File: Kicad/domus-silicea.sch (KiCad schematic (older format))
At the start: 6 parts, among them U1 MCP1640

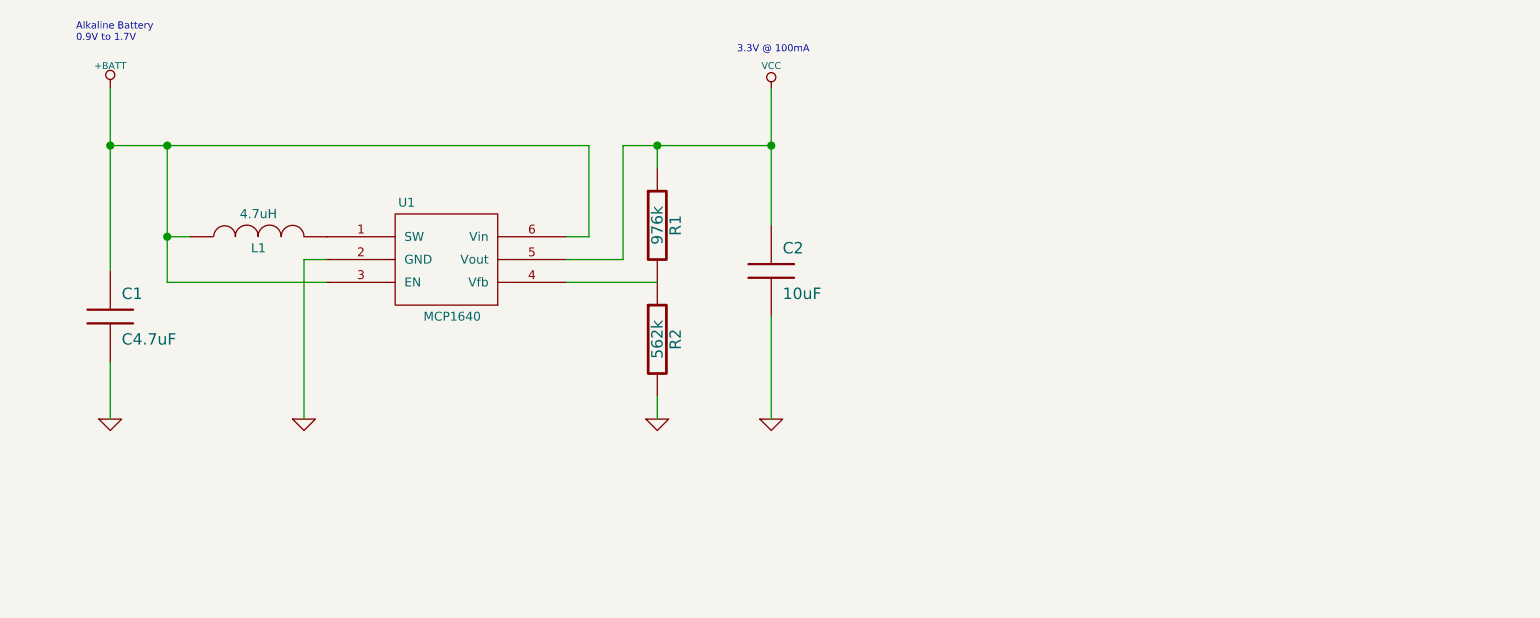
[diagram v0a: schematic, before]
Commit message: KiCad
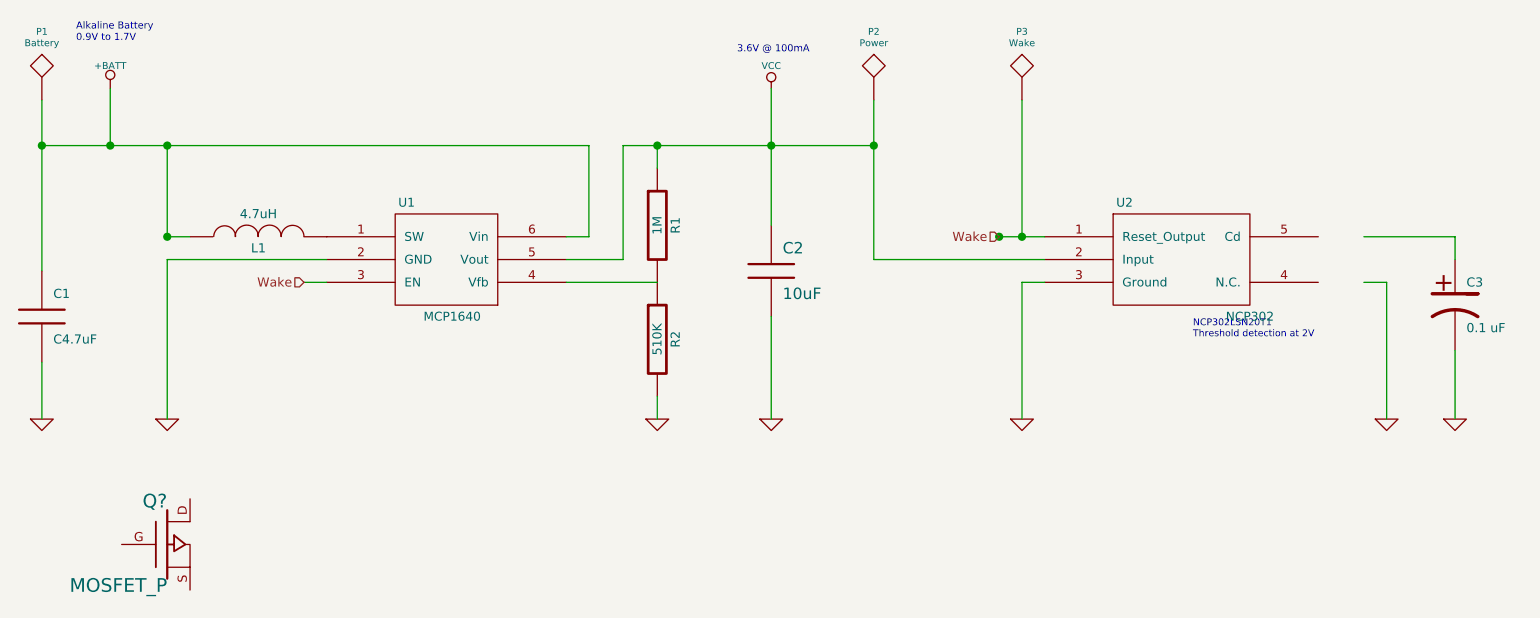
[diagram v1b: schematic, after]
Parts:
- added C3: 0.1 uF, symbol CP1
- added P1: Battery, symbol TST
- added P2: Power, symbol TST
- added P3: Wake, symbol TST
- added Q?: MOSFET_P, symbol MOSFET_P
- added U2: NCP302, symbol NCP302
- R1: value 976k -> 1M
- R2: value 562k -> 510K
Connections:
- net labels added: Wake
- wire segments 18 -> 30
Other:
- note added: "3.6V @ 100mA"
- note added: "NCP302LSN20T1\nThreshold detection at 2V"
- note removed: "3.3V @ 100mA"
- moved on the sheet: C1
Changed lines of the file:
@@
-EESchema Schematic File Version 2  date 2/13/2015 09:27:14
+EESchema Schematic File Version 2  date 2/16/2015 17:59:50
 LIBS:power
 LIBS:device
@@
 LIBS:valves
 LIBS:customComponents
-EELAYER 43  0
+LIBS:domus-silicea-cache
+EELAYER 25  0
 EELAYER END
 $Descr A4 11700 8267
@@
 Sheet 1 1
 Title "Silicino Prototype"
-Date "13 feb 2015"
+Date "16 feb 2015"
 Rev ""
 Comp ""
@@
 $EndDescr
 Wire Wire Line
-	1850 1700 1750 1700
-Wire Wire Line
-	1750 1700 1750 2400
-Wire Wire Line
-	900  2150 900  2400
+	1850 1700 1150 1700
+Connection ~ 600  1200
+Wire Wire Line
+	600  1750 600  1000
+Connection ~ 4900 1600
+Wire Wire Line
+	4900 1000 4900 1600
+Wire Wire Line
+	4250 1200 3150 1200
+Wire Wire Line
+	4250 1000 4250 1700
+Wire Wire Line
+	4250 1700 5000 1700
+Connection ~ 4800 1600
+Wire Wire Line
+	1750 1800 1850 1800
+Wire Wire Line
+	600  1200 3000 1200
+Wire Wire Line
+	4900 2400 4900 1800
+Wire Wire Line
+	4900 1800 5000 1800
+Wire Wire Line
+	6400 1600 6800 1600
+Wire Wire Line
+	6800 1600 6800 1700
+Wire Wire Line
+	1150 1700 1150 2400
+Wire Wire Line
+	600  2150 600  2400
 Connection ~ 3800 1200
 Wire Wire Line
@@
 Wire Wire Line
 	2900 1800 3300 1800
-Wire Wire Line
-	1850 1800 1150 1800
 Wire Wire Line
 	1250 1600 1150 1600
@@
 	3800 2400 3800 1950
 Connection ~ 1150 1200
-Wire Wire Line
-	1150 1800 1150 1200
 Connection ~ 900  1200
 Wire Wire Line
-	900  950  900  1750
-Wire Wire Line
 	2900 1600 3000 1600
 Wire Wire Line
 	3000 1600 3000 1200
 Wire Wire Line
-	3000 1200 900  1200
-Wire Wire Line
 	2900 1700 3150 1700
 Wire Wire Line
 	3150 1700 3150 1200
-Wire Wire Line
-	3150 1200 3800 1200
 Wire Wire Line
 	3300 1200 3300 1300
 Connection ~ 3300 1200
+Wire Wire Line
+	6800 2100 6800 2400
+Wire Wire Line
+	6500 2400 6500 1800
+Wire Wire Line
+	6500 1800 6400 1800
+Connection ~ 4250 1200
+Wire Wire Line
+	1150 1600 1150 1200
+Wire Wire Line
+	5000 1600 4800 1600
+Wire Wire Line
+	900  950  900  1200
+Text HLabel 1750 1800 0    40   Input ~ 0
+Wake
+Text HLabel 4800 1600 0    40   Input ~ 0
+Wake
+$Comp
+L MOSFET_P Q?
+U 1 1 54E2206B
+P 1150 2950
+F 0 "Q?" H 1150 3140 60  0000 R CNN
+F 1 "MOSFET_P" H 1150 2770 60  0000 R CNN
+	1    1150 2950
+	1    0    0    -1
+$EndComp
+Text Notes 5650 2050 0    30   ~ 0
+ NCP302LSN20T1\nThreshold detection at 2V
+$Comp
+L TST P1
+U 1 1 54E1F74F
+P 600 1000
+F 0 "P1" H 600 1300 30  0000 C CNN
+F 1 "Battery" H 600 1250 30  0000 C CNN
+	1    600  1000
+	1    0    0    -1
+$EndComp
+$Comp
+L TST P2
+U 1 1 54E1F73D
+P 4250 1000
+F 0 "P2" H 4250 1300 30  0000 C CNN
+F 1 "Power" H 4250 1250 30  0000 C CNN
+	1    4250 1000
+	1    0    0    -1
+$EndComp
+$Comp
+L TST P3
+U 1 1 54E1F729
+P 4900 1000
+F 0 "P3" H 4900 1300 30  0000 C CNN
+F 1 "Wake" H 4900 1250 30  0000 C CNN
+	1    4900 1000
+	1    0    0    -1
+$EndComp
+$Comp
+L CP1 C3
+U 1 1 54E1F57F
+P 6800 1900
+F 0 "C3" H 6850 2000 40  0000 L CNN
+F 1 "0.1 uF" H 6850 1800 40  0000 L CNN
+	1    6800 1900
+	1    0    0    -1
+$EndComp
+$Comp
+L GND #PWR?
+U 1 1 54E1F526
+P 6800 2400
+F 0 "#PWR?" H 6800 2400 30  0001 C CNN
+F 1 "GND" H 6800 2330 30  0001 C CNN
+	1    6800 2400
+	1    0    0    -1
+$EndComp
+$Comp
+L GND #PWR?
+U 1 1 54E1F521
+P 6500 2400
+F 0 "#PWR?" H 6500 2400 30  0001 C CNN
+F 1 "GND" H 6500 2330 30  0001 C CNN
+	1    6500 2400
+	1    0    0    -1
+$EndComp
+$Comp
+L GND #PWR?
+U 1 1 54E1F508
+P 4900 2400
+F 0 "#PWR?" H 4900 2400 30  0001 C CNN
+F 1 "GND" H 4900 2330 30  0001 C CNN
+	1    4900 2400
+	1    0    0    -1
+$EndComp
+$Comp
+L NCP302 U2
+U 1 1 54E1F4D1
+P 5350 1700
+F 0 "U2" H 5350 1950 39  0000 C CNN
+F 1 "NCP302" H 5900 1450 39  0000 C CNN
+	1    5350 1700
+	1    0    0    -1
+$EndComp
 $Comp
 L MCP1640 U1
@@
 Alkaline Battery\n0.9V to 1.7V\n
 Text Notes 3650 800  0    31   ~ 0
-3.3V @ 100mA
+3.6V @ 100mA
 $Comp
 L VCC #PWR?
@@
 L GND #PWR?
 U 1 1 54DDAFB7
-P 900 2400
-F 0 "#PWR?" H 900 2400 30  0001 C CNN
-F 1 "GND" H 900 2330 30  0001 C CNN
-	1    900  2400
+P 600 2400
+F 0 "#PWR?" H 600 2400 30  0001 C CNN
+F 1 "GND" H 600 2330 30  0001 C CNN
+	1    600  2400
 	1    0    0    -1
 $EndComp
@@
 L C C1
 U 1 1 54DDABB5
-P 900 1950
-F 0 "C1" H 950 2050 50  0000 L CNN
-F 1 "C4.7uF" H 950 1850 50  0000 L CNN
-	1    900  1950
+P 600 1950
+F 0 "C1" H 650 2050 40  0000 L CNN
+F 1 "C4.7uF" H 650 1850 40  0000 L CNN
+	1    600  1950
 	1    0    0    -1
 $EndComp
@@
 U 1 1 54DDAB61
 P 3300 2050
-F 0 "R2" V 3380 2050 50  0000 C CNN
-F 1 "562k" V 3300 2050 50  0000 C CNN
+F 0 "R2" V 3380 2050 40  0000 C CNN
+F 1 "510K" V 3300 2050 40  0000 C CNN
 	1    3300 2050
 	1    0    0    -1
@@
 U 1 1 54DDAB5A
 P 3300 1550
-F 0 "R1" V 3380 1550 50  0000 C CNN
-F 1 "976k" V 3300 1550 50  0000 C CNN
+F 0 "R1" V 3380 1550 40  0000 C CNN
+F 1 "1M" V 3300 1550 40  0000 C CNN
 	1    3300 1550
 	1    0    0    -1
@@
 L GND #PWR?
 U 1 1 54DDA9D6
-P 1750 2400
-F 0 "#PWR?" H 1750 2400 30  0001 C CNN
-F 1 "GND" H 1750 2330 30  0001 C CNN
-	1    1750 2400
-	1    0    0    -1
-$EndComp
+P 1150 2400
+F 0 "#PWR?" H 1150 2400 30  0001 C CNN
+F 1 "GND" H 1150 2330 30  0001 C CNN
+	1    1150 2400
+	1    0    0    -1
+$EndComp

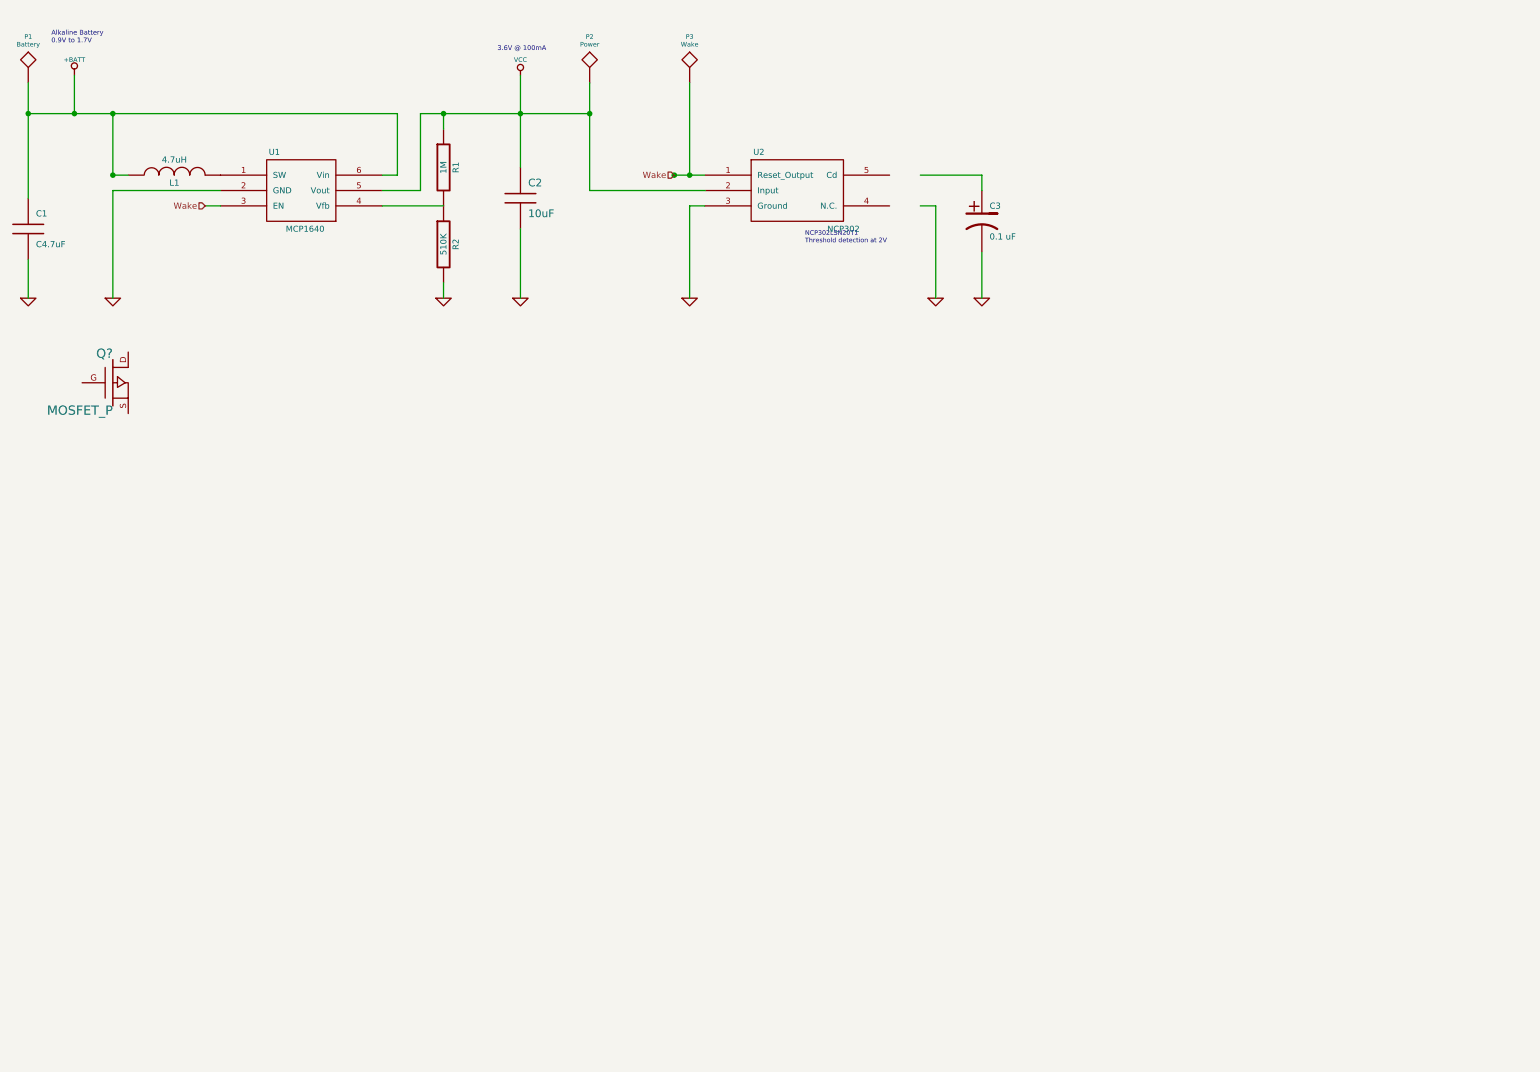
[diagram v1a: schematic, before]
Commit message: Raspbmc
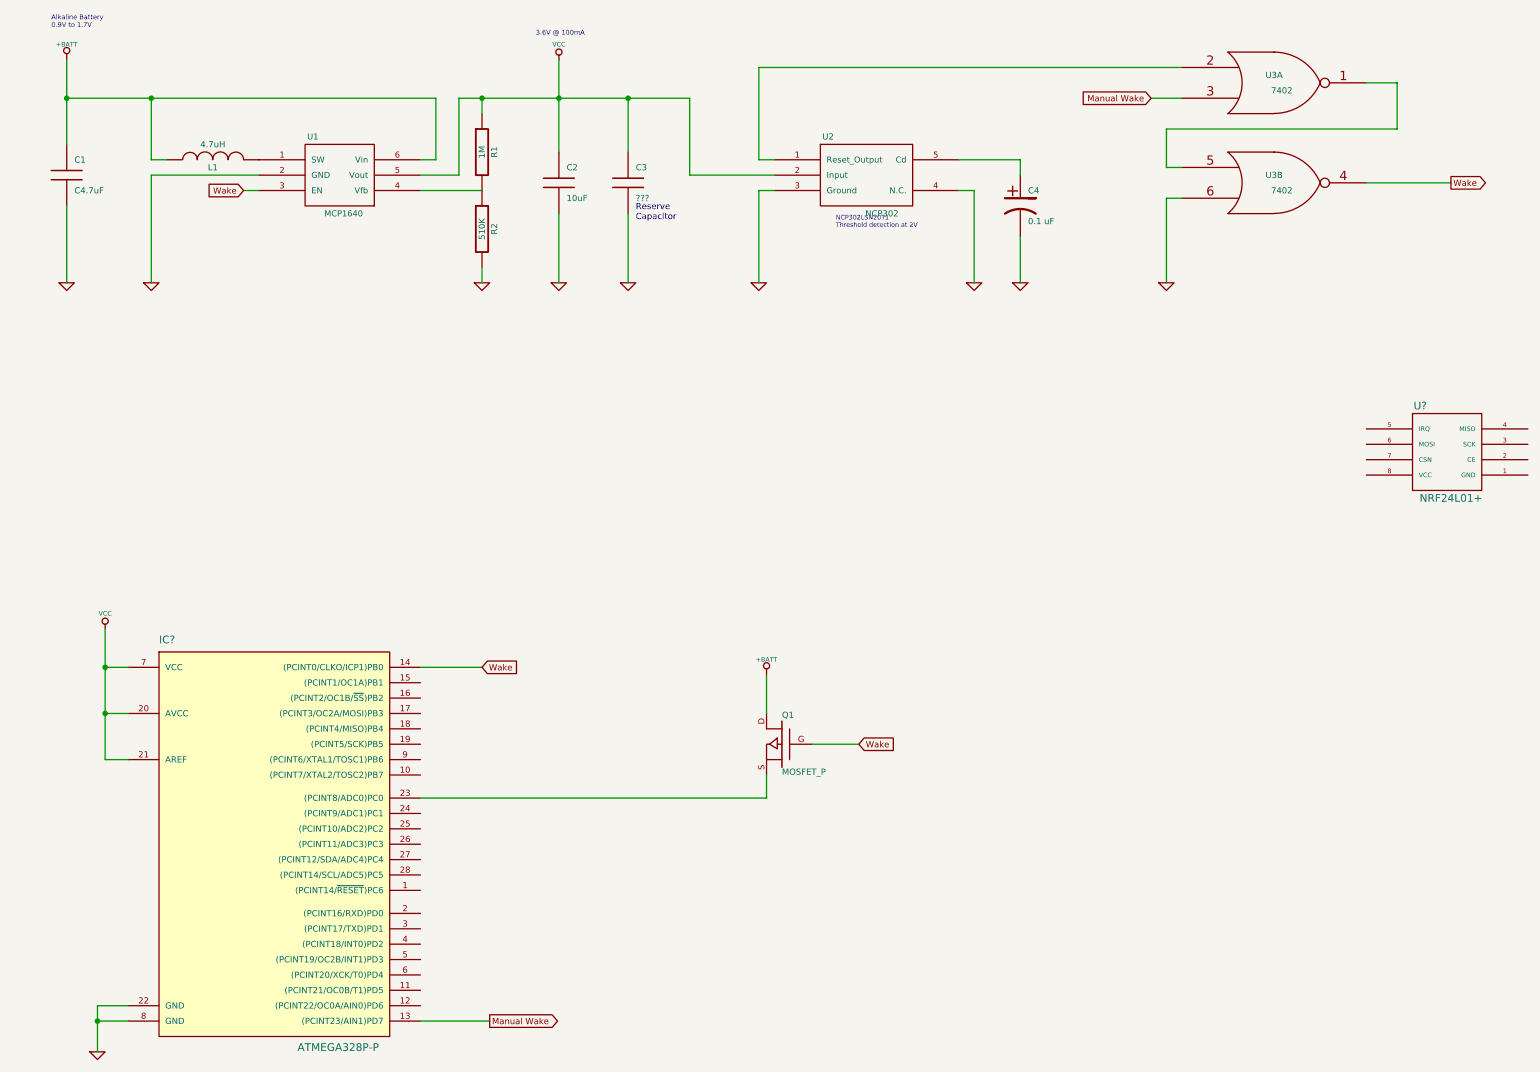
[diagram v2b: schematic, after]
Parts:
- removed P1: Battery, symbol TST
- removed P2: Power, symbol TST
- removed P3: Wake, symbol TST
- added C3: ???, symbol C
- added IC?: ATMEGA328P-P, DIL28, symbol ATMEGA328P-P
- added U3: 7402, symbol 7402
- added U?: NRF24L01+, symbol NRF24L01+
- gave numbers to parts that had none: 1
- renumbered C3 to C4
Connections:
- net labels added: Manual Wake
- wire segments 30 -> 54
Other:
- note added: "Reserve\nCapacitor"
- moved on the sheet: C1, C2, C4, L1, Q1, R1, R2, U1
